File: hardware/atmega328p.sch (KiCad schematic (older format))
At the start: 23 parts, among them J401 USART, J402 DISABLE, U401 ATMEGA328P-PU, Y401 16MHz

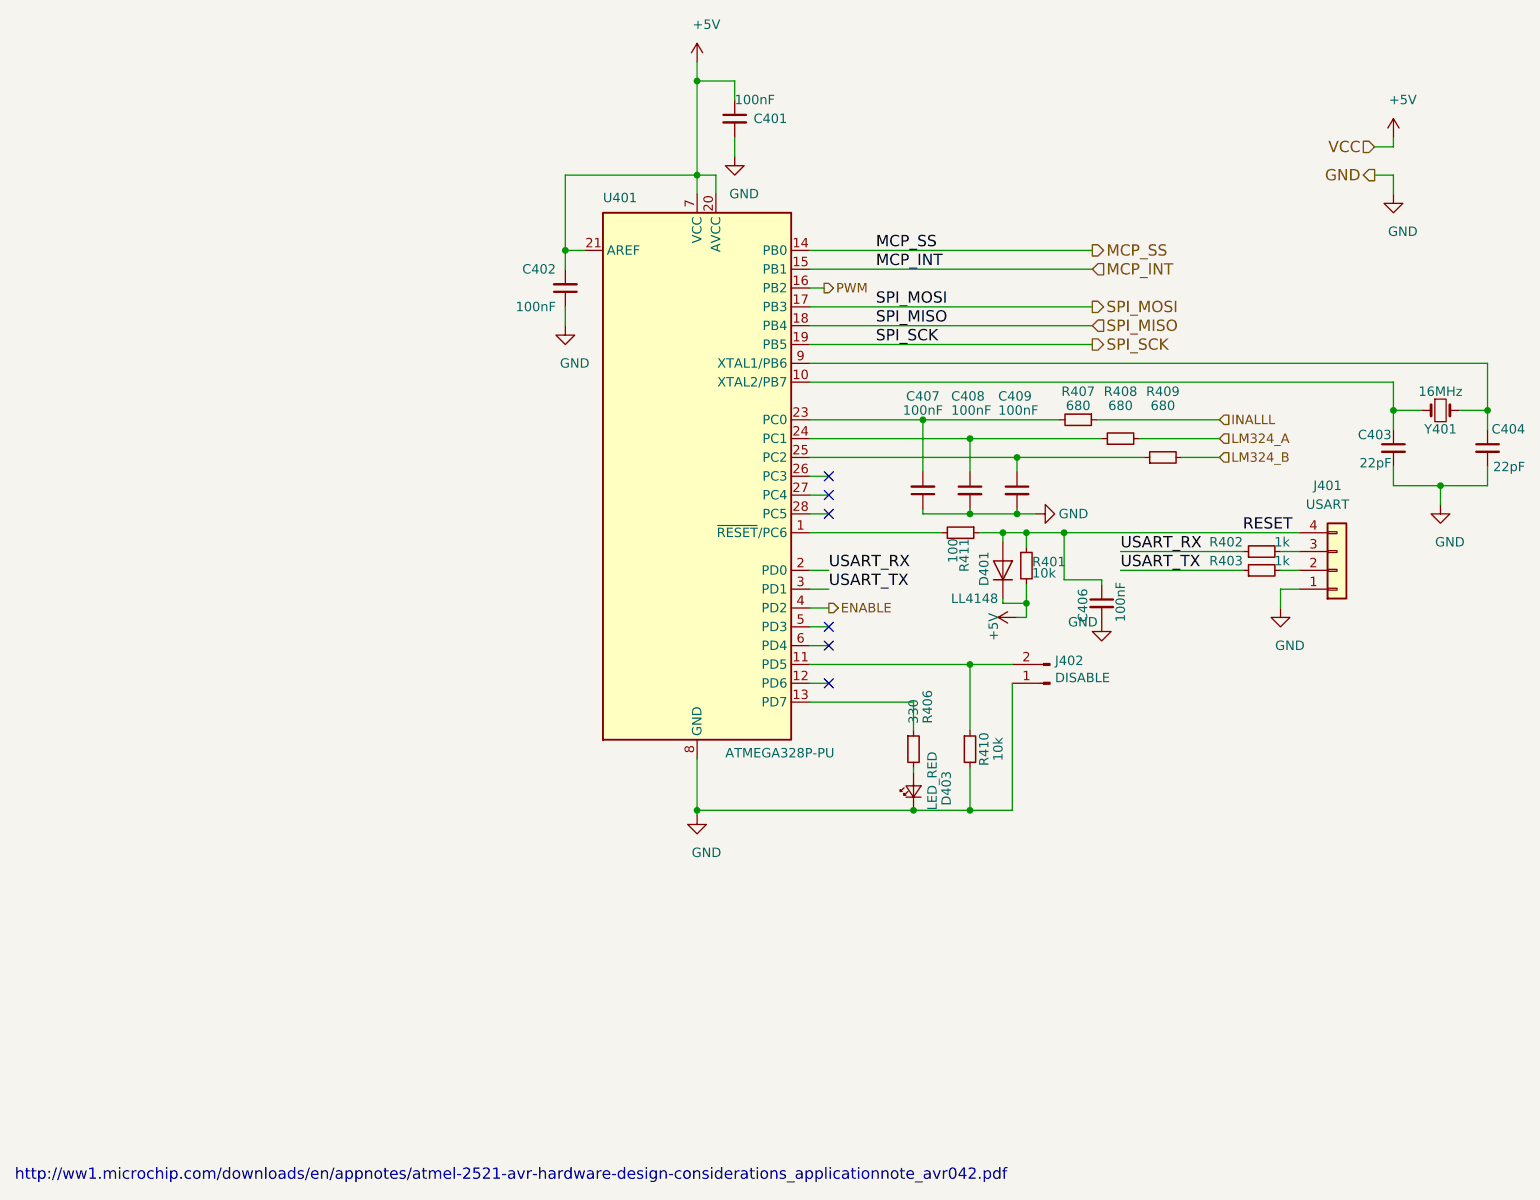
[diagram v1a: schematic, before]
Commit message: Some fixes, ready for heat transfering
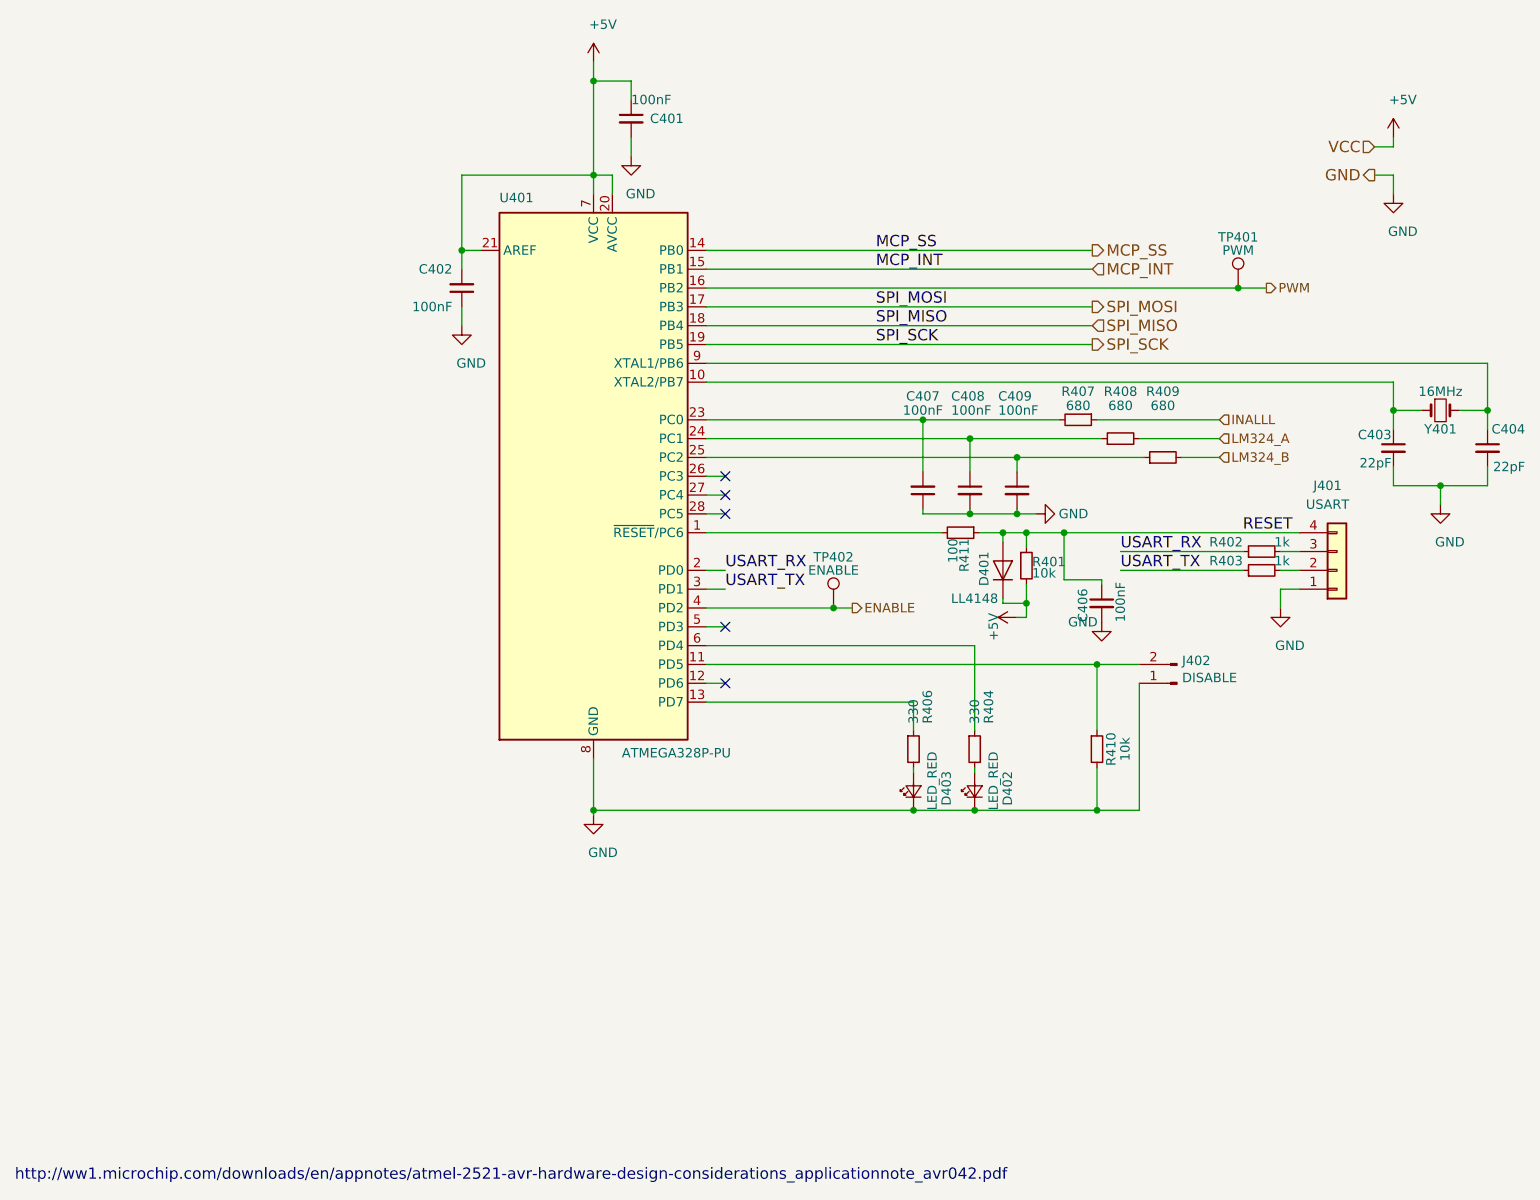
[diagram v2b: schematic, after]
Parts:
- added D402: LED_RED, LED_SMD:LED_0805_2012Metric_Pad1.15x1.40mm_HandSolder, symbol Device:LED_Small
- added R404: 330, Resistor_SMD:R_0805_2012Metric_Pad1.15x1.40mm_HandSolder, symbol Device:R_Small
- added TP401: PWM, TestPoint:TestPoint_Pad_2.0x2.0mm, symbol Connector:TestPoint
- added TP402: ENABLE, TestPoint:TestPoint_Pad_2.0x2.0mm, symbol Connector:TestPoint
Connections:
- net ENABLE: now also TP402.1
- net GND: now also D402.1 (K)
- net PWM: now also TP401.1
- net at U401.6 (PD4): now also R404.1
- new net: D402.2 (A), R404.2
- no-connect marks 6 -> 5
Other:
- moved on the sheet: C401, C402, J402, R410, U401
